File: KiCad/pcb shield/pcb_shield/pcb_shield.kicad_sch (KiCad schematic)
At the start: 3 parts, among them J1 Raspberry Pi Zero, U1 BOB-09056

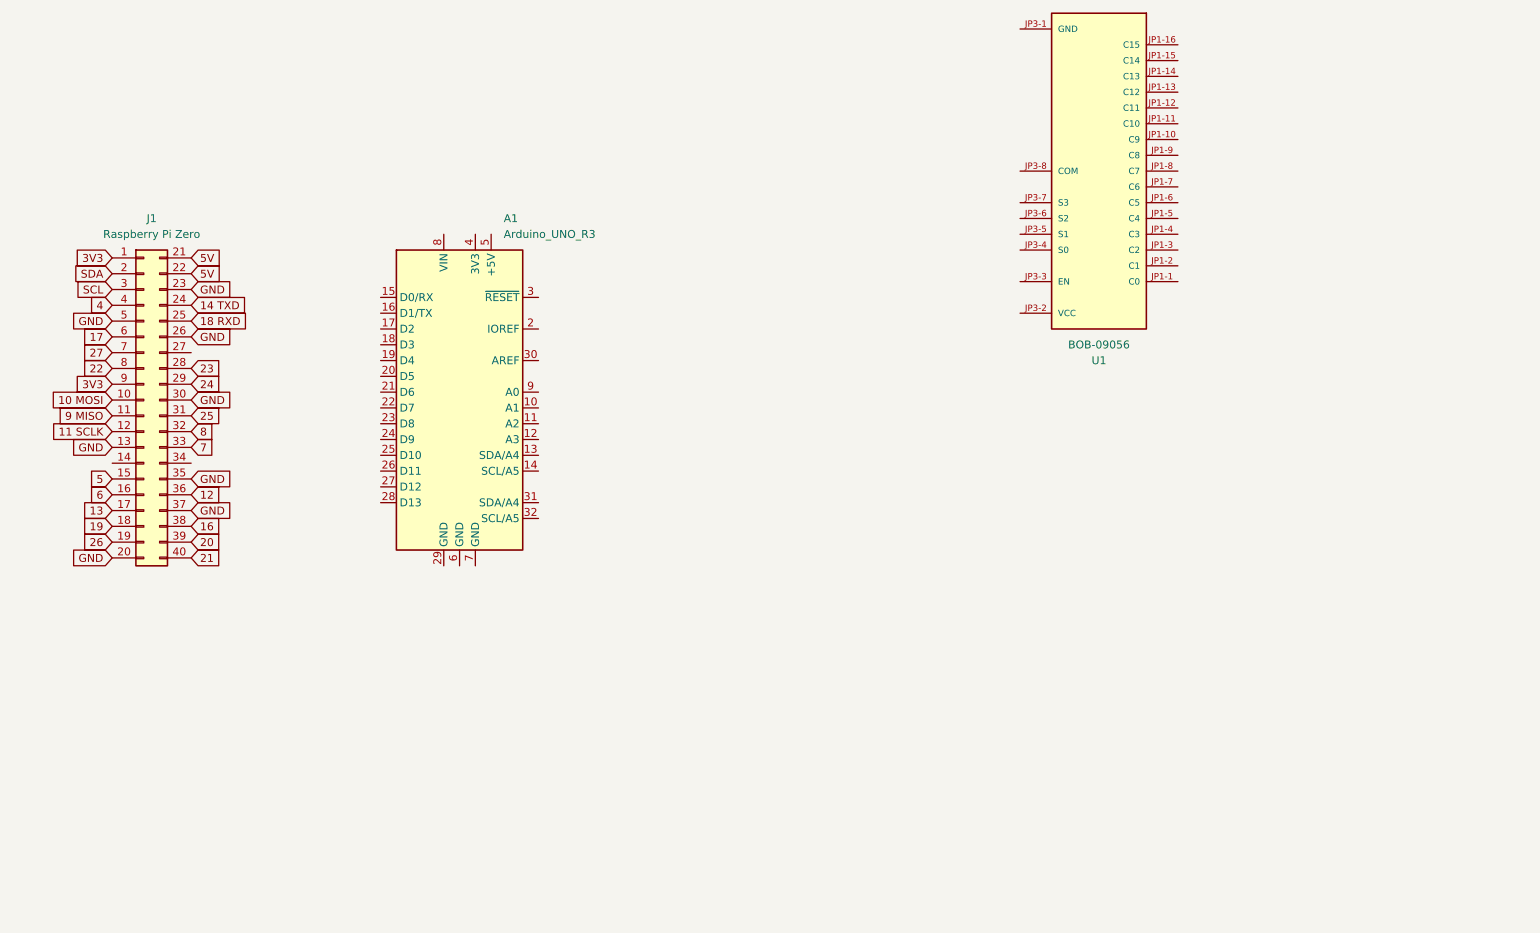
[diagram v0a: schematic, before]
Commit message: add main parts
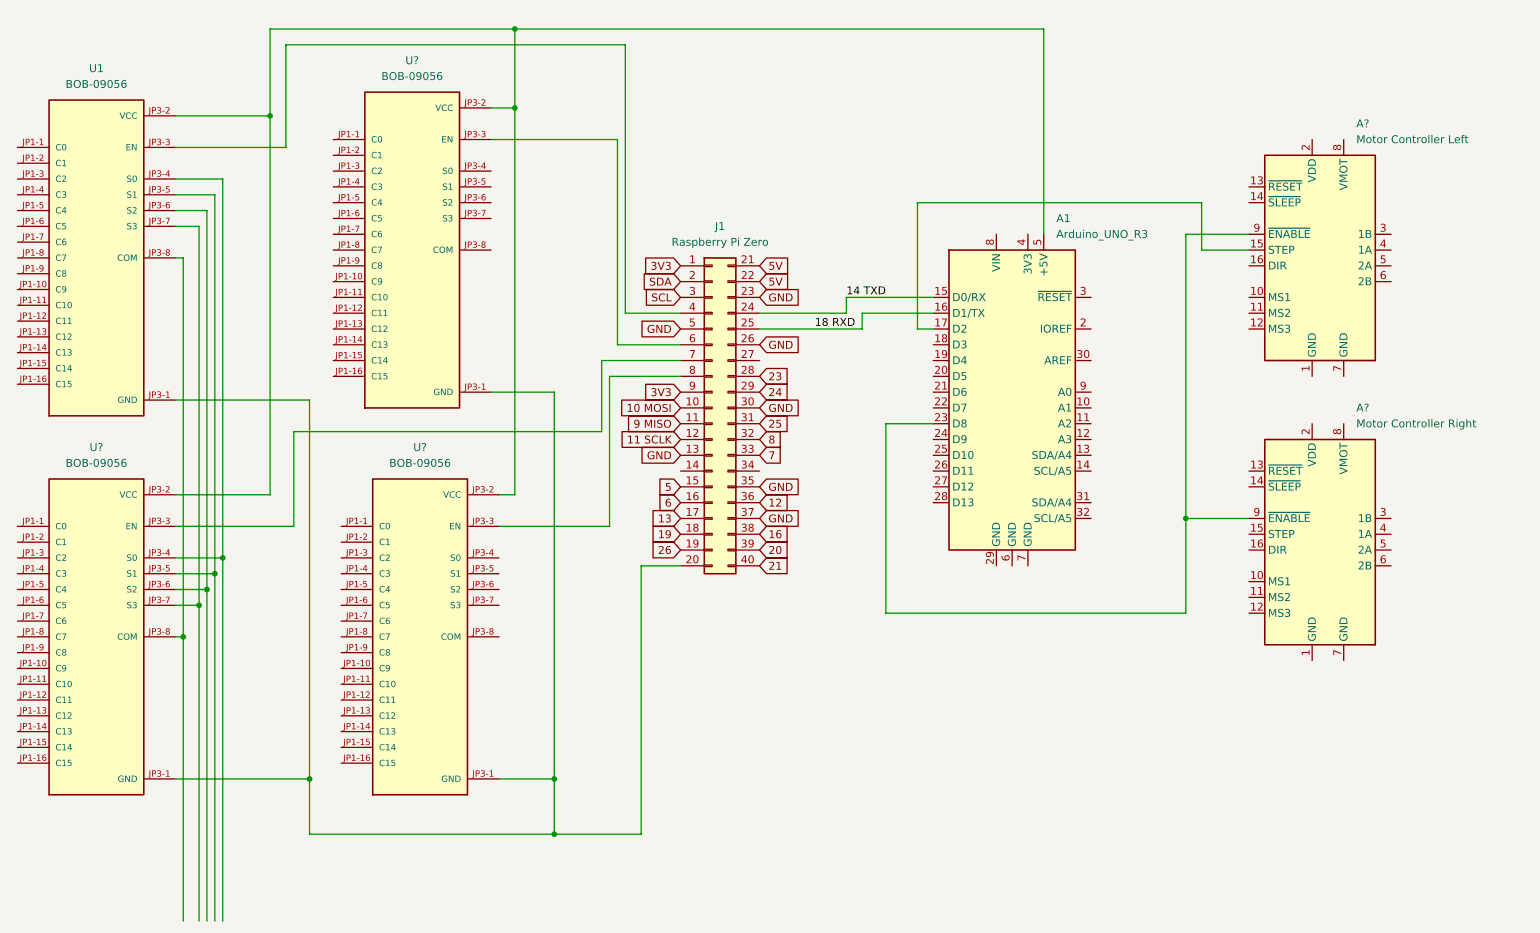
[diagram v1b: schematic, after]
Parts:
- added A?: Motor Controller Left, Module:Pololu_Breakout-16_15.2x20.3mm, symbol Driver_Motor:Pololu_Breakout_A4988
- added A?: Motor Controller Right, Module:Pololu_Breakout-16_15.2x20.3mm, symbol Driver_Motor:Pololu_Breakout_A4988
- added U? (x3): BOB-09056, BOB-09056:MODULE_BOB-09056, symbol BOB-09056:BOB-09056
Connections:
- net 4 is gone; now on an unnamed net: J1.4 (Pin_4)
- net 14 TXD: now also A1.15 (D0/RX)
- net 18 RXD: now also A1.16 (D1/TX)
- net GND: no longer J1.20 (Pin_20)
- net at U1.JP3-1 (GND): now also J1.20 (Pin_20), U?.JP3-1 (GND), U?.JP3-1 (GND), U?.JP3-1 (GND)
- net at U1.JP3-2 (VCC): now also A1.5 (+5V), U?.JP3-2 (VCC), U?.JP3-2 (VCC), U?.JP3-2 (VCC)
- net at U1.JP3-4 (S0): now also U?.JP3-4 (S0)
- net at U1.JP3-5 (S1): now also U?.JP3-5 (S1)
- net at U1.JP3-6 (S2): now also U?.JP3-6 (S2)
- net at U1.JP3-7 (S3): now also U?.JP3-7 (S3)
- net at U1.JP3-8 (COM): now also U?.JP3-8 (COM)
- net at A1.17 (D2): now also A?.15 (STEP)
- net at A1.23 (D8): now also A?.9 (~{ENABLE}), A?.9 (~{ENABLE})
- net 17: no longer names the net of J1.6 (Pin_6)
- net 17: now also U?.JP3-3 (EN)
- net 22: no longer names the net of J1.8 (Pin_8)
- net 22: now also U?.JP3-3 (EN)
- net 27: no longer names the net of J1.7 (Pin_7)
- net 27: now also U?.JP3-3 (EN)
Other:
- moved on the sheet: A1, J1, U1

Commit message: start with pcb
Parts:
- added C1, C2: C, Capacitor_THT:CP_Radial_D5.0mm_P2.50mm, symbol Device:C
- added J1, J2, J3, J4, J5, J6, J7, J8: (no value), Connector_PinHeader_2.54mm:PinHeader_2x04_P2.54mm_Vertical, symbol Connector_Generic:Conn_02x04_Counter_Clockwise
- added J10, J11: Motor Conn, Connector_PinHeader_2.54mm:PinHeader_1x04_P2.54mm_Vertical, symbol Connector_Generic:Conn_01x04
- added J12: Endstop X, Connector_PinHeader_2.54mm:PinHeader_1x02_P2.54mm_Vertical, symbol Connector_Generic:Conn_01x02
- added J13: Endstop Y, Connector_PinHeader_2.54mm:PinHeader_1x02_P2.54mm_Vertical, symbol Connector_Generic:Conn_01x02
- added J14: Barrel_Jack, symbol Connector:Barrel_Jack
- added J9: E_Magnet, Connector_PinHeader_2.54mm:PinHeader_1x02_P2.54mm_Vertical, symbol Connector_Generic:Conn_01x02
- added Q1: TIP120, Package_TO_SOT_THT:TO-220-3_Vertical, symbol Transistor_BJT:TIP120
- gave numbers to parts that had none: 5
- renumbered J1 to A1, A1 to A2
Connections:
- net 5V: now also U1.JP3-2 (VCC), U2.JP3-2 (VCC), U3.JP3-2 (VCC), U4.JP3-2 (VCC)
- net at U3.JP1-1 (C0): now also J5.1 (Pin_1)
- net at U3.JP1-10 (C9): now also J6.8 (Pin_8)
- net at U3.JP1-11 (C10): now also J6.2 (Pin_2)
- net at U3.JP1-12 (C11): now also J6.7 (Pin_7)
- net at U3.JP1-13 (C12): now also J6.3 (Pin_3)
- net at U3.JP1-14 (C13): now also J6.6 (Pin_6)
- net at U3.JP1-15 (C14): now also J6.4 (Pin_4)
- net at U3.JP1-16 (C15): now also J6.5 (Pin_5)
- net at U3.JP1-2 (C1): now also J5.8 (Pin_8)
- net at U3.JP1-3 (C2): now also J5.2 (Pin_2)
- net at U3.JP1-4 (C3): now also J5.7 (Pin_7)
- net at U3.JP1-5 (C4): now also J5.3 (Pin_3)
- net at U3.JP1-6 (C5): now also J5.6 (Pin_6)
- net at U3.JP1-7 (C6): now also J5.4 (Pin_4)
- net at U3.JP1-8 (C7): now also J5.5 (Pin_5)
- net at U3.JP1-9 (C8): now also J6.1 (Pin_1)
- net at U3.JP3-4 (S0): now also U1.JP3-4 (S0), U2.JP3-4 (S0)
- net at U3.JP3-5 (S1): now also U1.JP3-5 (S1), U2.JP3-5 (S1)
- net at U3.JP3-6 (S2): now also U1.JP3-6 (S2), U2.JP3-6 (S2)
- net at U3.JP3-7 (S3): now also U1.JP3-7 (S3), U2.JP3-7 (S3)
- net at U3.JP3-8 (COM): now also U1.JP3-8 (COM), U2.JP3-8 (COM)
- net at U1.JP1-1 (C0): now also J1.1 (Pin_1)
- net at U1.JP1-10 (C9): now also J2.8 (Pin_8)
- net at U1.JP1-11 (C10): now also J2.2 (Pin_2)
- net at U1.JP1-12 (C11): now also J2.7 (Pin_7)
- net at U1.JP1-13 (C12): now also J2.3 (Pin_3)
- net at U1.JP1-14 (C13): now also J2.6 (Pin_6)
- net at U1.JP1-15 (C14): now also J2.4 (Pin_4)
- net at U1.JP1-16 (C15): now also J2.5 (Pin_5)
- net at U1.JP1-2 (C1): now also J1.8 (Pin_8)
- net at U1.JP1-3 (C2): now also J1.2 (Pin_2)
- net at U1.JP1-4 (C3): now also J1.7 (Pin_7)
- net at U1.JP1-5 (C4): now also J1.3 (Pin_3)
- net at U1.JP1-6 (C5): now also J1.6 (Pin_6)
- net at U1.JP1-7 (C6): now also J1.4 (Pin_4)
- net at U1.JP1-8 (C7): now also J1.5 (Pin_5)
- net at U1.JP1-9 (C8): now also J2.1 (Pin_1)
- net at A3.1 (GND): now also A2.7 (GND), A4.1 (GND), J12.2 (Pin_2), J13.2 (Pin_2)
- net at A3.16 (DIR): now also A2.20 (D5)
- net at A3.2 (VDD): now also A2.5 (+5V), A4.2 (VDD)
- net at A3.3 (1B): now also J10.1 (Pin_1)
- net at A3.4 (1A): now also J10.2 (Pin_2)
- net at A3.5 (2A): now also J10.3 (Pin_3)
- net at A3.6 (2B): now also J10.4 (Pin_4)
- net at A3.7 (GND): now also A4.7 (GND), C1.2, C2.2, J14.1, J9.1 (Pin_1)
- net at A3.8 (VMOT): now also A4.8 (VMOT), C1.1, C2.1, J14.2, Q1.2 (C)
- net at A4.15 (STEP): now also A2.18 (D3)
- net at A4.16 (DIR): now also A2.21 (D6)
- net at A4.3 (1B): now also J11.1 (Pin_1)
- net at A4.4 (1A): now also J11.2 (Pin_2)
- net at A4.5 (2A): now also J11.3 (Pin_3)
- net at A4.6 (2B): now also J11.4 (Pin_4)
- net at U4.JP1-1 (C0): now also J7.1 (Pin_1)
- net at U4.JP1-10 (C9): now also J8.8 (Pin_8)
- net at U4.JP1-11 (C10): now also J8.2 (Pin_2)
- net at U4.JP1-12 (C11): now also J8.7 (Pin_7)
- net at U4.JP1-13 (C12): now also J8.3 (Pin_3)
- net at U4.JP1-14 (C13): now also J8.6 (Pin_6)
- net at U4.JP1-15 (C14): now also J8.4 (Pin_4)
- net at U4.JP1-16 (C15): now also J8.5 (Pin_5)
- net at U4.JP1-2 (C1): now also J7.8 (Pin_8)
- net at U4.JP1-3 (C2): now also J7.2 (Pin_2)
- net at U4.JP1-4 (C3): now also J7.7 (Pin_7)
- net at U4.JP1-5 (C4): now also J7.3 (Pin_3)
- net at U4.JP1-6 (C5): now also J7.6 (Pin_6)
- net at U4.JP1-7 (C6): now also J7.4 (Pin_4)
- net at U4.JP1-8 (C7): now also J7.5 (Pin_5)
- net at U4.JP1-9 (C8): now also J8.1 (Pin_1)
- net at U2.JP1-1 (C0): now also J3.1 (Pin_1)
- net at U2.JP1-10 (C9): now also J4.8 (Pin_8)
- net at U2.JP1-11 (C10): now also J4.2 (Pin_2)
- net at U2.JP1-12 (C11): now also J4.7 (Pin_7)
- net at U2.JP1-13 (C12): now also J4.3 (Pin_3)
- net at U2.JP1-14 (C13): now also J4.6 (Pin_6)
- net at U2.JP1-15 (C14): now also J4.4 (Pin_4)
- net at U2.JP1-16 (C15): now also J4.5 (Pin_5)
- net at U2.JP1-2 (C1): now also J3.8 (Pin_8)
- net at U2.JP1-3 (C2): now also J3.2 (Pin_2)
- net at U2.JP1-4 (C3): now also J3.7 (Pin_7)
- net at U2.JP1-5 (C4): now also J3.3 (Pin_3)
- net at U2.JP1-6 (C5): now also J3.6 (Pin_6)
- net at U2.JP1-7 (C6): now also J3.4 (Pin_4)
- net at U2.JP1-8 (C7): now also J3.5 (Pin_5)
- net at U2.JP1-9 (C8): now also J4.1 (Pin_1)
- net at A2.24 (D9): now also J12.1 (Pin_1)
- net at A2.25 (D10): now also J13.1 (Pin_1)
- net at A2.26 (D11): now also Q1.1 (B)
- new net: J9.2 (Pin_2), Q1.3 (E)
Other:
- moved on the sheet: A1, A2, A3, A4, U1, U2, U3, U4
